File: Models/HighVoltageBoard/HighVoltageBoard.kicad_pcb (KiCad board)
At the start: 2 copper layers, 1 part

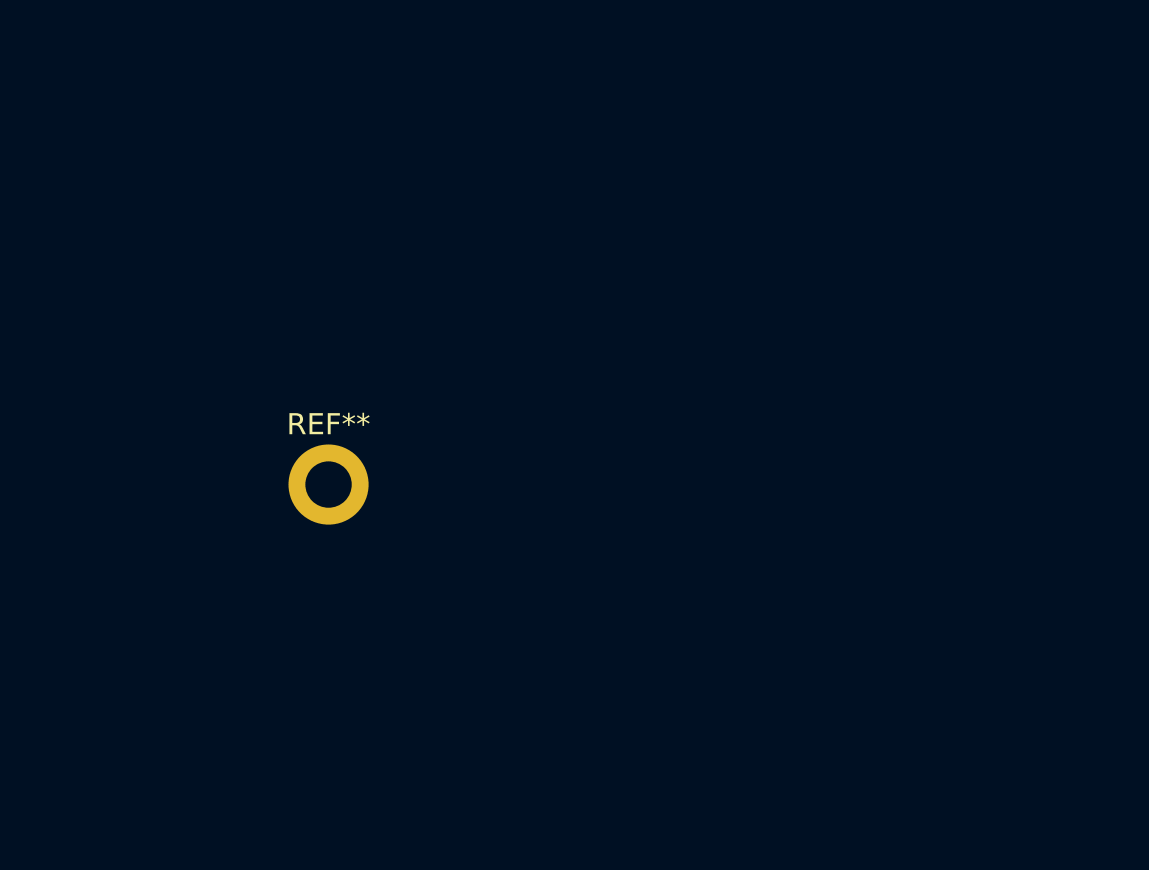
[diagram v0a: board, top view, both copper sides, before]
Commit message: Finished THT footprints
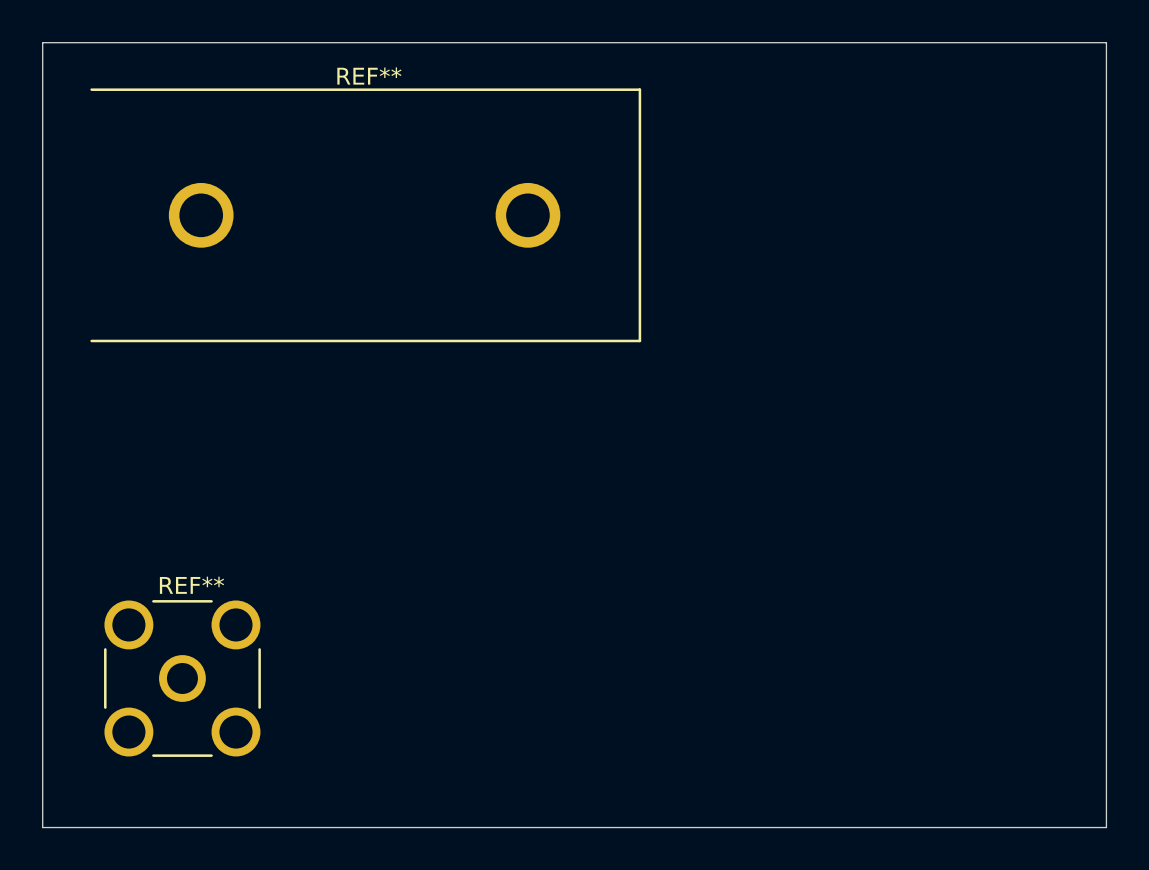
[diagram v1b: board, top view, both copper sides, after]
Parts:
- removed the REF** at (152.9, 114.2)
- added REF**: RFPC-SMA27-F, Connector_Custom:RFPC-SMA27-F, F.Cu at (145.9, 123.3)
- added REF**: Multicomp_24.243, Connector_Custom:Multicomp_24.243, F.Cu at (154.6, 101.4)
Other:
- board outline added: 50.5 x 37.2 mm
